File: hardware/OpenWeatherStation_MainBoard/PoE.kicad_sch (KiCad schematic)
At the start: 1 part, among them J1 RJ45_LED_Shielded

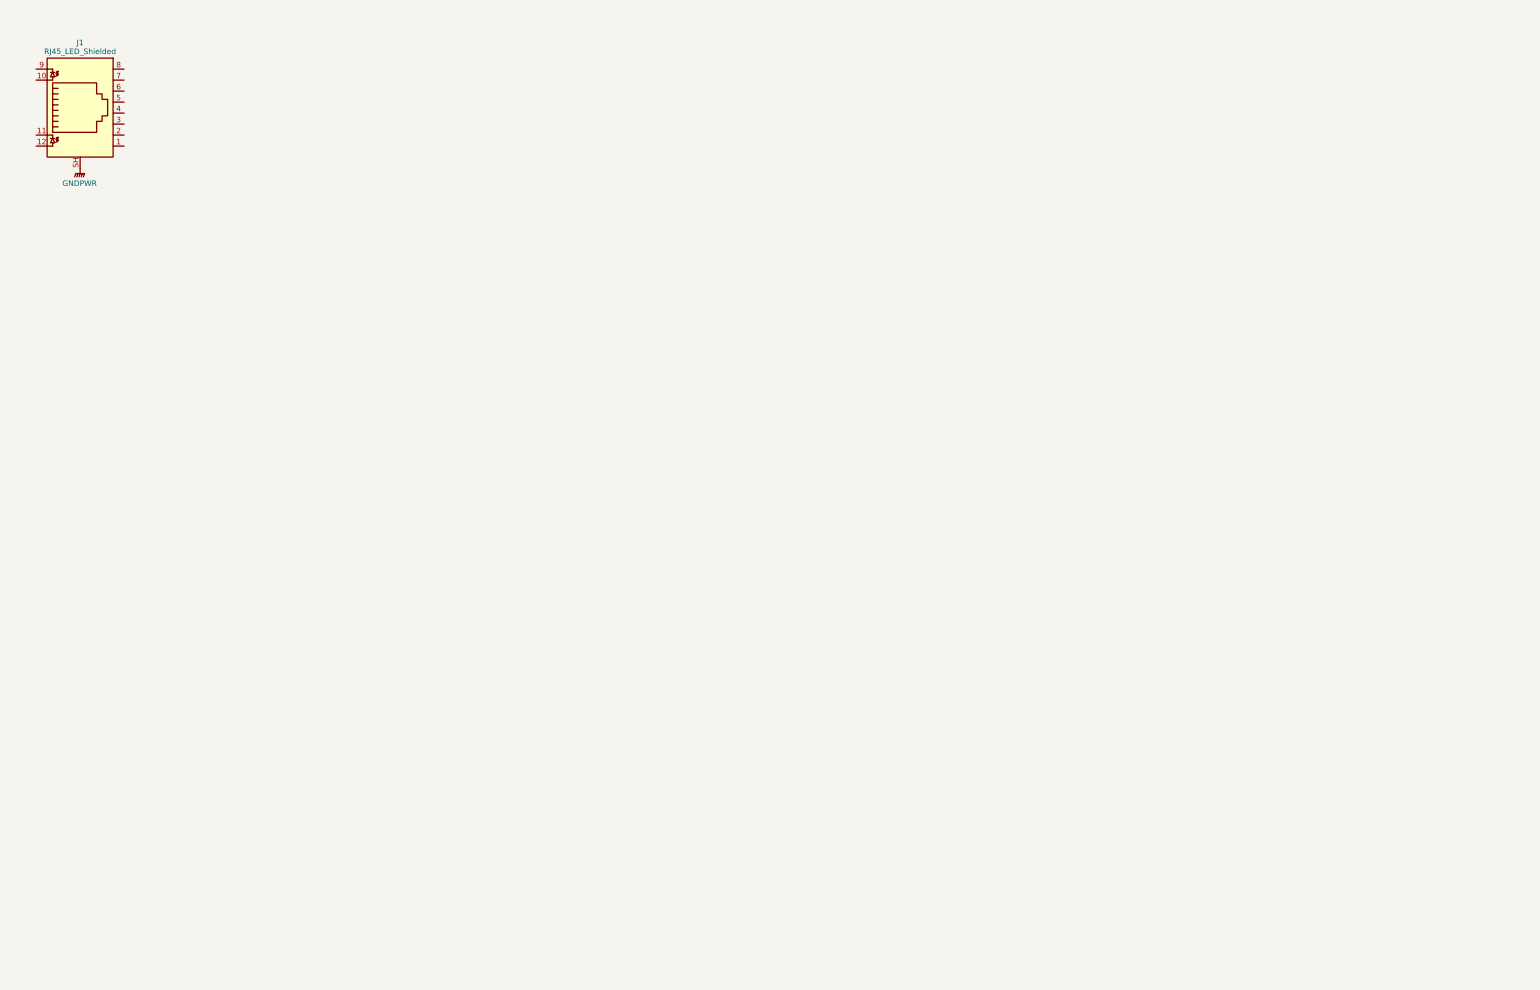
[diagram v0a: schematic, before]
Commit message: clean
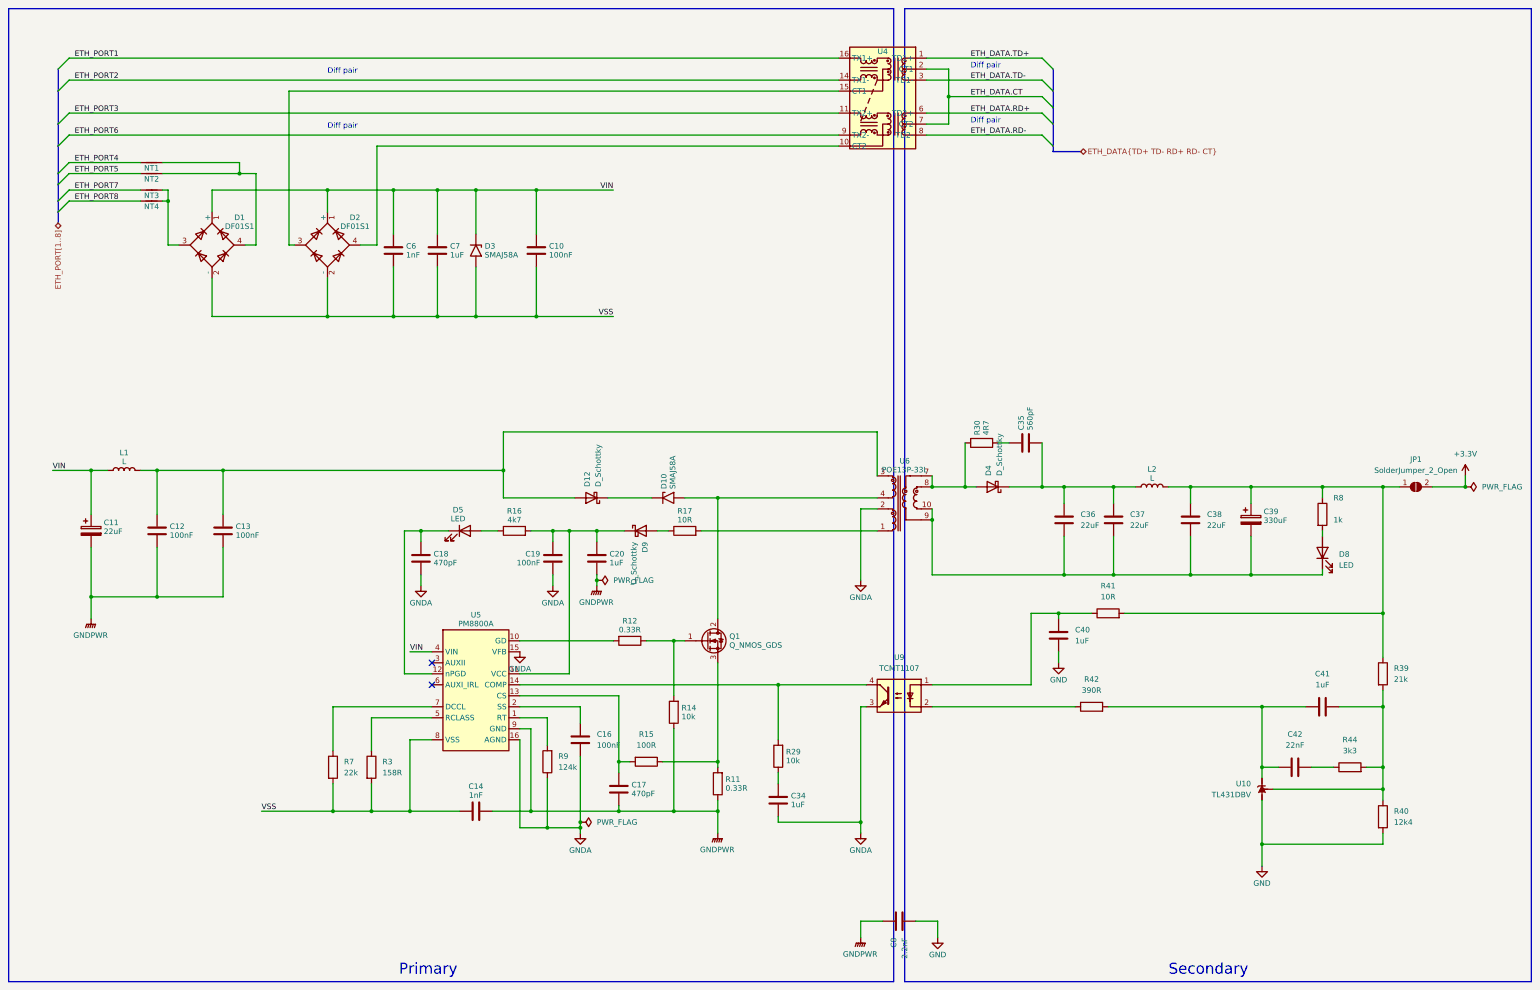
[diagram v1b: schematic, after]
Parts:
- removed J1: RJ45_LED_Shielded, symbol Connector:RJ45_LED_Shielded
- added C10, C12, C13, C16, C19: 100nF, Capacitor_SMD:C_0603_1608Metric, symbol Device:C
- added C11: 22uF, Capacitor_SMD:CP_Elec_5x3, symbol Device:C_Polarized
- added C14, C6: 1nF, Capacitor_SMD:C_0603_1608Metric, symbol Device:C
- added C17, C18: 470pF, Capacitor_SMD:C_0603_1608Metric, symbol Device:C
- added C20, C34, C40, C41, C7: 1uF, Capacitor_SMD:C_0603_1608Metric, symbol Device:C
- added C35: 560pF, Capacitor_SMD:C_0603_1608Metric, symbol Device:C
- added C36, C37, C38: 22uF, Capacitor_SMD:C_0603_1608Metric, symbol Device:C
- added C39: 330uF, Capacitor_SMD:CP_Elec_5x3, symbol Device:C_Polarized
- added C42: 22nF, Capacitor_SMD:C_0603_1608Metric, symbol Device:C
- added C8: 2.2nF, Capacitor_SMD:C_0603_1608Metric, symbol Device:C
- added D1, D2: DF01S1, Diode_SMD:Diode_Bridge_OnSemi_SDIP-4L, symbol Diode_Bridge:DF01S1
- added D10, D3: SMAJ58A, Diode_SMD:D_SMA, symbol Diode:SMAJ58A
- added D12, D9: D_Schottky, Diode_SMD:D_1206_3216Metric, symbol Device:D_Schottky
- added D4: D_Schottky, Diode_SMD:D_PowerDI-5, symbol Device:D_Schottky
- added D5, D8: LED, LED_THT:LED_D3.0mm, symbol Device:LED
- added JP1: SolderJumper_2_Open, Jumper:SolderJumper-2_P1.3mm_Open_RoundedPad1.0x1.5mm, symbol Jumper:SolderJumper_2_Open
- added L1, L2: L, Inductor_SMD:L_1206_3216Metric, symbol Device:L
- added NT1, NT2, NT3, NT4: NetTie_2, NetTie:NetTie-2_SMD_Pad0.5mm, symbol Device:NetTie_2
- added Q1: Q_NMOS_GDS, Package_TO_SOT_SMD:TO-252-2, symbol Device:Q_NMOS_GDS
- added R11: 0.33R, Resistor_SMD:R_1206_3216Metric, symbol Device:R
- added R12: 0.33R, Resistor_SMD:R_0603_1608Metric, symbol Device:R
- added R14, R29: 10k, Resistor_SMD:R_0603_1608Metric, symbol Device:R
- added R15: 100R, Resistor_SMD:R_0603_1608Metric, symbol Device:R
- added R16: 4k7, Resistor_SMD:R_0603_1608Metric, symbol Device:R
- added R17, R41: 10R, Resistor_SMD:R_0603_1608Metric, symbol Device:R
- added R3: 158R, Resistor_SMD:R_0603_1608Metric, symbol Device:R
- added R30: 4R7, Resistor_SMD:R_0603_1608Metric, symbol Device:R
- added R39: 21k, Resistor_SMD:R_0603_1608Metric, symbol Device:R
- added R40: 12k4, Resistor_SMD:R_0603_1608Metric, symbol Device:R
- added R42: 390R, Resistor_SMD:R_0603_1608Metric, symbol Device:R
- added R44: 3k3, Resistor_SMD:R_0603_1608Metric, symbol Device:R
- added R7: 22k, Resistor_SMD:R_0603_1608Metric, symbol Device:R
- added R8: 1k, Resistor_SMD:R_0603_1608Metric, symbol Device:R
- added R9: 124k, Resistor_SMD:R_0603_1608Metric, symbol Device:R
- added U10: TL431DBV, Package_TO_SOT_SMD:SOT-23-5, symbol Reference_Voltage:TL431DBV
- added U4: ~, Transformer_SMD:Transformer_Ethernet_Wuerth_749013011A, symbol New_Library:SM13126PEL
- added U5: PM8800A, Package_SO:HTSSOP-16-1EP_4.4x5mm_P0.65mm_EP3x3mm, symbol New_Library:PM8800A
- added U6: POE13P-33L, Library:SM13117EL, symbol New_Library:POE13P-33L
- added U9: TCMT1107, Package_SO:SOP-4_4.4x2.6mm_P1.27mm, symbol Isolator:TCMT1107
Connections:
- net GNDPWR: now also C11.2, C12.2, C13.2, C14.2, C17.2, C20.2, C8.1, R11.1, R14.1, U5.9 (GND)
- new net: R9.2, U5.1 (RT)
- new net: C41.1, R39.2, R40.1, R44.2, U10.4 (REF)
- new net: C40.2, R41.1, U9.1
- new net: C38.2, C39.1, JP1.1 (A), L2.2, R39.1, R41.2, R8.1
- new net: C19.1, C20.1, D9.1 (K), R16.2, U5.11 (VCC)
- new net: D9.2 (A), R17.1
- new net: Q1.1 (G), R12.1, R14.2
- new net: C34.1, R29.1
- new net: R29.2, U5.14 (COMP), U9.4
- new net: C36.1, C37.1, C38.1, C39.2, D8.1 (K), U6.10, U6.9
- new net: D8.2 (A), R8.2
- new net: C12.1, C13.1, D12.2 (A), L1.2, U6.3
- new net: R42.1, U9.2
- new net: Q1.3 (S), R11.2, R15.1
- new net: C17.1, R15.2, U5.13 (CS)
- new net: D10.2 (A2), Q1.2 (D), U6.4
- new net: C35.1, R30.1
- new net: C35.2, C36.2, C37.2, D4.1 (K), L2.1
- new net: C42.1, R44.1
- new net: C41.2, C42.2, R42.2, U10.3 (K)
- new net: R17.2, U6.1
- new net: D4.2 (A), R30.2, U6.7, U6.8
- new net: C16.1, U5.2 (SS)
- new net: D10.1 (A1), D12.1 (K)
- new net: D2.4, U4.10 (CT2)
- new net: D2.3, U4.15 (CT1)
- new net: D1.4, NT1.2, NT2.2
- new net: D1.3, NT3.2, NT4.2
- new net: C18.1, D5.1 (K), U5.12 (nPGD)
- new net: R12.2, U5.10 (GD)
- new net: R3.1, U5.5 (RCLASS)
- new net: R7.1, U5.7 (DCCL)
- new net: D5.2 (A), R16.1
- new net +3.3V: JP1.2 (B)
- new net ETH_DATA.CT: U4.2 (CT1), U4.7 (CT2)
- new net ETH_DATA.RD+: U4.6 (TD2+)
- new net ETH_DATA.RD-: U4.8 (TD2-)
- new net ETH_DATA.TD+: U4.1 (TD1+)
- new net ETH_DATA.TD-: U4.3 (TD1-)
- new net ETH_PORT1: U4.16 (TX1+)
- new net ETH_PORT2: U4.14 (TX1-)
- new net ETH_PORT3: U4.11 (TX2+)
- new net ETH_PORT4: NT1.1
- new net ETH_PORT5: NT2.1
- new net ETH_PORT6: U4.9 (TX2-)
- new net ETH_PORT7: NT3.1
- new net ETH_PORT8: NT4.1
- new net GND: C40.1, C8.2, R40.2, U10.5 (A)
- new net GNDA: C16.2, C18.2, C19.2, C34.2, R9.1, U5.15 (VFB), U5.16 (AGND), U6.2, U9.3
- new net VIN: C10.1, C11.1, C6.1, C7.1, D1.1 (+), D2.1 (+), D3.1 (A1), L1.1, U5.4 (VIN)
- new net VSS: C10.2, C14.1, C6.2, C7.2, D1.2 (-), D2.2 (-), D3.2 (A2), R3.2, R7.2, U5.8 (VSS)
- no-connect marks 0 -> 2
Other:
- note added: "Diff pair"
- note added: "Primary"
- note added: "Secondary"
